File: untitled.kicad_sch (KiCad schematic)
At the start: 3 parts, among them J3 DB25_Pins, J4 DB25_Socket, J7 Conn_02x10_Odd_Even

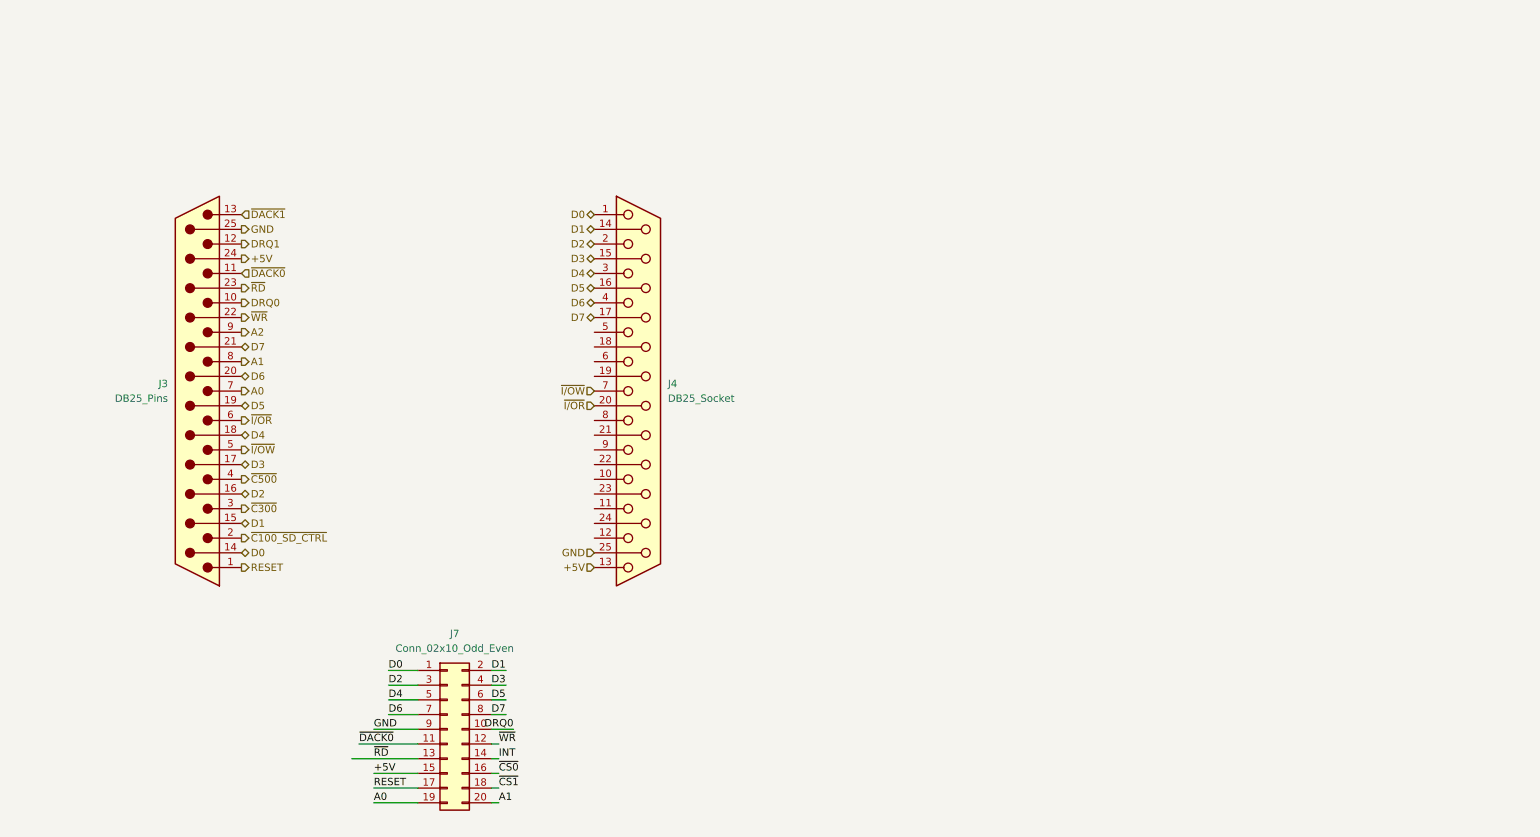
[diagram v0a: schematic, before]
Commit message: Update untitled.kicad_sch
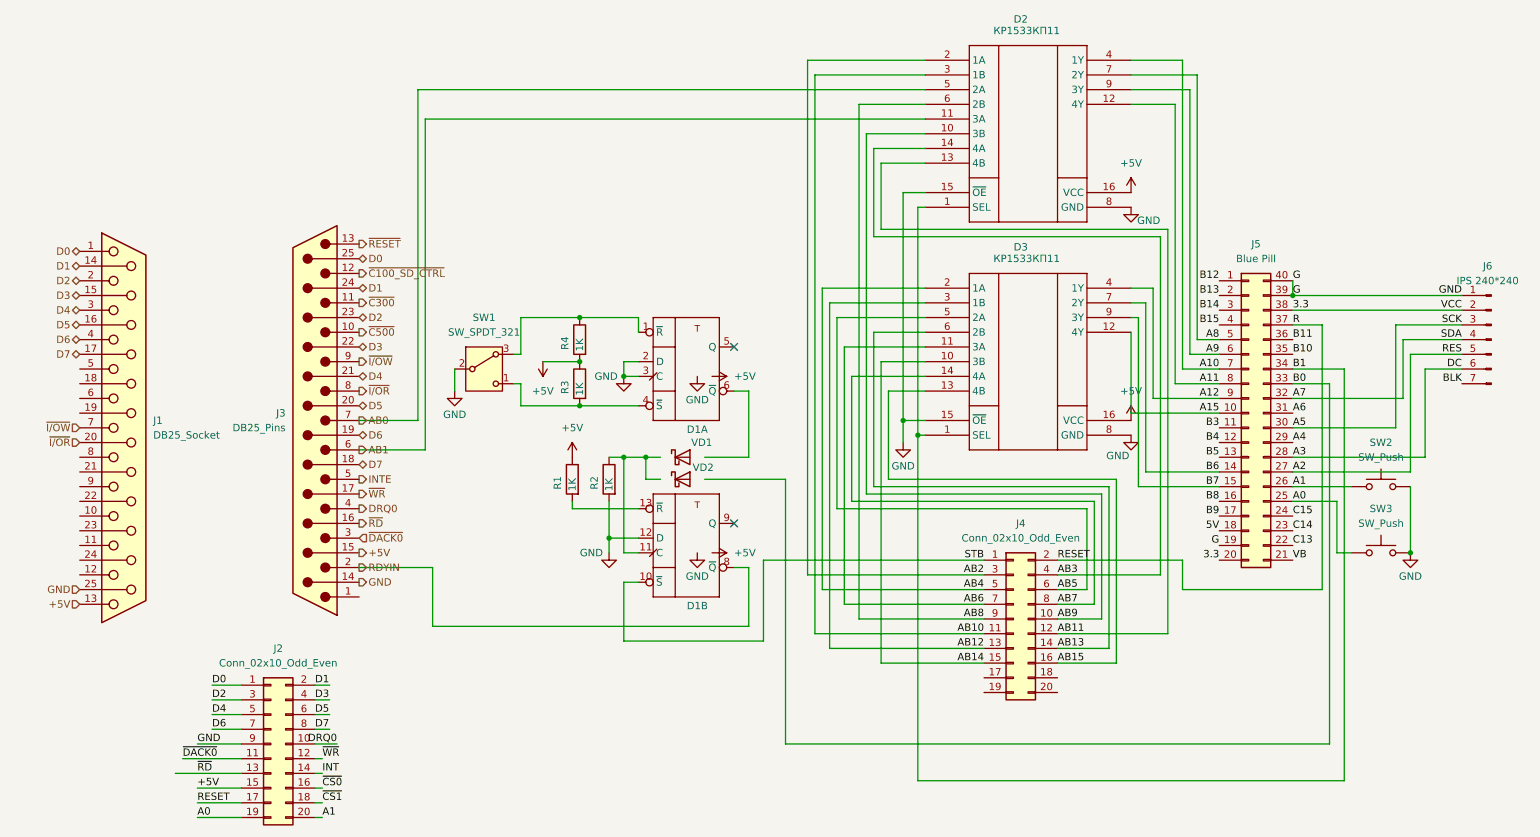
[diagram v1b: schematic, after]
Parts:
- added D1: 74HC74N, Package_DIP:DIP-14_W7.62mm_Socket, symbol VGA_Sync-altium-import:root_0_74HC74N_*
- added D2, D3: КР1533КП11, Package_DIP:DIP-16_W7.62mm, symbol Pico-altium-import:root_0_KR1533KP11_*
- added J4: Conn_02x10_Odd_Even, Connector_PinHeader_1.00mm:PinHeader_2x10_P1.00mm_Vertical, symbol Connector_Generic:Conn_02x10_Odd_Even
- added J5: Blue Pill, symbol Connector_Generic:Conn_02x20_Counter_Clockwise
- added J6: IPS 240*240, symbol Connector:Conn_01x07_Pin
- added R1, R2, R3, R4: 1K, Resistor_THT:R_Axial_DIN0207_L6.3mm_D2.5mm_P5.08mm_Vertical, symbol Device:R
- added SW1: SW_SPDT_321, symbol Switch:SW_SPDT_321
- added SW2, SW3: SW_Push, symbol Switch:SW_Push
- added VD1, VD2: 1N4148, Diode_THT:D_DO-34_SOD68_P2.54mm_Vertical_AnodeUp, symbol Diode:BAT43
- renumbered J4 to J1, J7 to J2
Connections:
- net DRQ1 is gone; now on net ~{C100_SD_CTRL}: J3.12
- net +5V: now also J3.15 (P15), D1.14 (VCC), D1.14 (VCC), D2.16 (VCC), D3.16 (VCC), J5.20 (Pin_20), J5.38 (Pin_38), J6.2 (Pin_2), R1.1, R3.1, R4.2; no longer J3.24 (P24)
- net A0: now also J5.25 (Pin_25), SW3.1; no longer J3.7
- net A1: now also J5.26 (Pin_26), SW2.1; no longer J3.8
- net A2: now also J5.27 (Pin_27), J6.5 (Pin_5); no longer J3.9
- net D0: now also J3.25 (P25); no longer J3.14 (P14)
- net D1: now also J3.24 (P24); no longer J3.15 (P15)
- net D2: now also J3.23 (P23); no longer J3.16 (P16)
- net D3: now also J3.22 (P22); no longer J3.17 (P17)
- net D4: now also J3.21 (P21); no longer J3.18 (P18)
- net D5: now also J3.20 (P20); no longer J3.19 (P19)
- net D6: now also J3.19 (P19); no longer J3.20 (P20)
- net D7: now also J3.18 (P18); no longer J3.21 (P21)
- net DRQ0: now also J3.4; no longer J3.10
- net GND: now also J3.14 (P14), D1.12 (D), D1.2 (D), D1.3 (C), D1.7 (GND), D1.7 (GND), D2.15 (~{OE}), D2.8 (GND), D3.15 (~{OE}), D3.8 (GND), J5.19 (Pin_19), J5.39 (Pin_39), J5.40 (Pin_40), J6.1 (Pin_1), R2.2, SW1.2 (B), SW2.2, SW3.2; no longer J3.25 (P25)
- net ~{C100_SD_CTRL}: no longer J3.2
- net ~{C300}: now also J3.11; no longer J3.3
- net ~{C500}: now also J3.10; no longer J3.4
- net ~{DACK0}: now also J3.3; no longer J3.11
- net ~{I/OR}: now also J3.8; no longer J3.6
- net ~{I/OW}: now also J3.9; no longer J3.5
- net ~{RD}: now also J3.16 (P16); no longer J3.23 (P23)
- net ~{WR}: now also J3.17 (P17); no longer J3.22 (P22)
- net RESET: no longer names the net of J3.1
- net RESET: no longer J2.17 (Pin_17)
- net ~{DACK1} renamed ~{RESET}
- new net: D1.11 (C), R2.1
- new net: D1.13 (~{R}), R1.2
- new net: D1.1 (~{R}), R4.1, SW1.3 (A)
- new net: D1.4 (~{S}), R3.2, SW1.1 (C)
- new net 5V: J5.18 (Pin_18)
- new net A10: D2.4 (1Y), J5.7 (Pin_7)
- new net A11: D2.12 (4Y), J5.8 (Pin_8)
- new net A12: D3.4 (1Y), J5.9 (Pin_9)
- new net A15: D3.12 (4Y), J5.10 (Pin_10)
- new net A3: J5.28 (Pin_28), J6.6 (Pin_6)
- new net A4: J5.29 (Pin_29)
- new net A5: J5.30 (Pin_30), J6.3 (Pin_3)
- new net A6: J5.31 (Pin_31)
- new net A7: J5.32 (Pin_32), J6.4 (Pin_4)
- new net A8: D2.7 (2Y), J5.5 (Pin_5)
- new net A9: D2.9 (3Y), J5.6 (Pin_6)
- new net AB0: D2.5 (2A), J3.7
- new net AB1: D2.11 (3A), J3.6
- new net AB10: D2.3 (1B), J4.11 (Pin_11)
- new net AB11: D2.13 (4B), J4.12 (Pin_12)
- new net AB12: D3.3 (1B), J4.13 (Pin_13)
- new net AB13: D3.6 (2B), J4.14 (Pin_14)
- new net AB14: D3.10 (3B), J4.15 (Pin_15)
- new net AB15: D3.13 (4B), J4.16 (Pin_16)
- new net AB2: D2.2 (1A), J4.3 (Pin_3)
- new net AB3: D2.14 (4A), J4.4 (Pin_4)
- new net AB4: D3.2 (1A), J4.5 (Pin_5)
- new net AB5: D3.5 (2A), J4.6 (Pin_6)
- new net AB6: D3.11 (3A), J4.7 (Pin_7)
- new net AB7: D3.14 (4A), J4.8 (Pin_8)
- new net AB8: D2.6 (2B), J4.9 (Pin_9)
- new net AB9: D2.10 (3B), J4.10 (Pin_10)
- new net B0: J5.33 (Pin_33)
- new net B1: D2.1 (SEL), D3.1 (SEL), J5.34 (Pin_34)
- new net B10: J5.35 (Pin_35)
- new net B11: J5.36 (Pin_36)
- new net B12: J5.1 (Pin_1)
- new net B13: J5.2 (Pin_2)
- new net B14: J5.3 (Pin_3)
- new net B15: J5.4 (Pin_4)
- new net B3: J5.11 (Pin_11)
- new net B4: J5.12 (Pin_12)
- new net B5: J5.13 (Pin_13)
- new net B6: D3.7 (2Y), J5.14 (Pin_14)
- new net B7: D3.9 (3Y), J5.15 (Pin_15)
- new net B8: J5.16 (Pin_16)
- new net B9: J5.17 (Pin_17)
- new net BLK: J6.7 (Pin_7)
- new net C13: J5.22 (Pin_22)
- new net C14: J5.23 (Pin_23)
- new net C15: J5.24 (Pin_24)
- new net INTE: J3.5
- new net R: J2.17 (Pin_17), J4.2 (Pin_2), J5.37 (Pin_37)
- new net RDYIN: D1.8 (~{Q}), J3.2
- new net STB: D1.10 (~{S}), J4.1 (Pin_1)
- new net VB: J5.21 (Pin_21)
- no-connect marks 0 -> 2
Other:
- moved on the sheet: J1, J2, J3
